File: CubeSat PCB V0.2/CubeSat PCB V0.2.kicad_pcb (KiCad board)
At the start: 2 copper layers, 34.4 x 65.5 mm, 8 parts, among them J1 Raspberry_Pi_2_3, J2 Encoder Connector, J3 LSM9DS1, J4 XT60PW-M, J5 Conn_01x03_Female, J6 XT60PW-F, SW1 SW_DPDT_x2, U1 MP1584EN

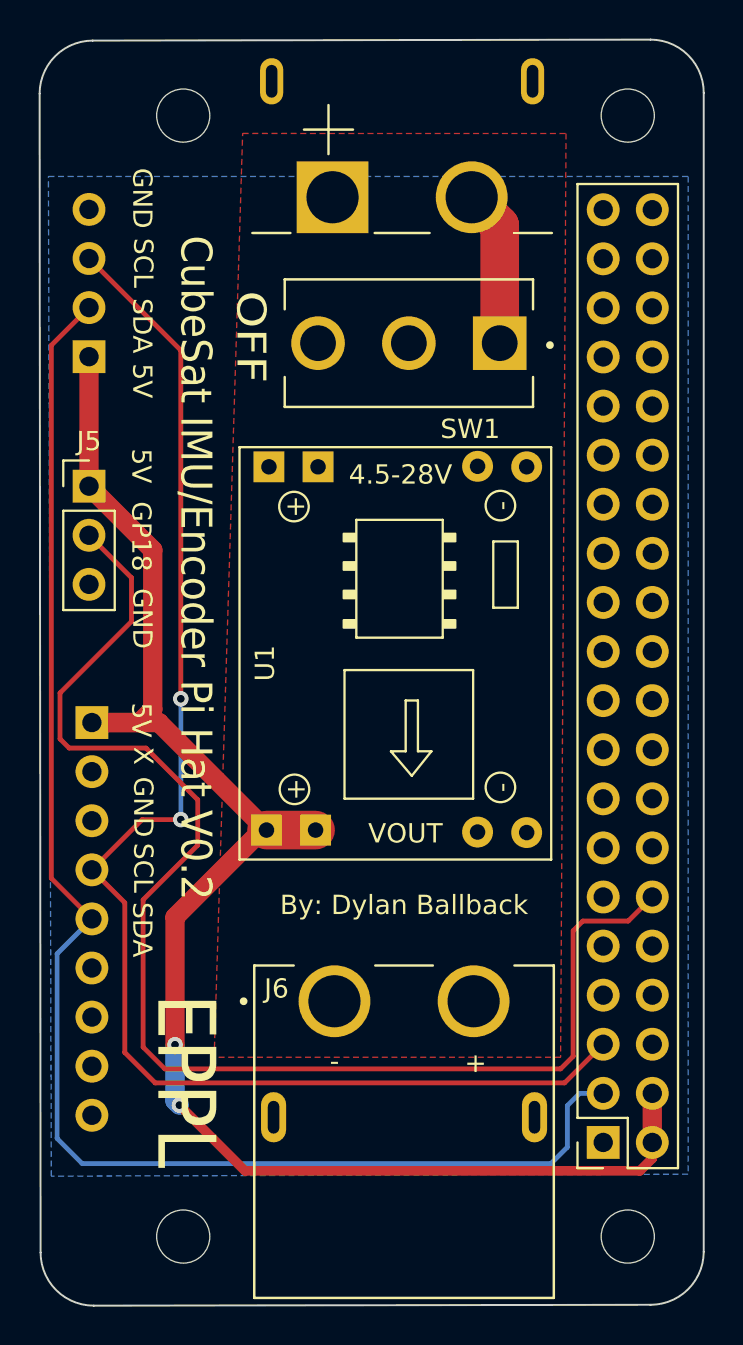
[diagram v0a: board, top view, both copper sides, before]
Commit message: Add files via upload
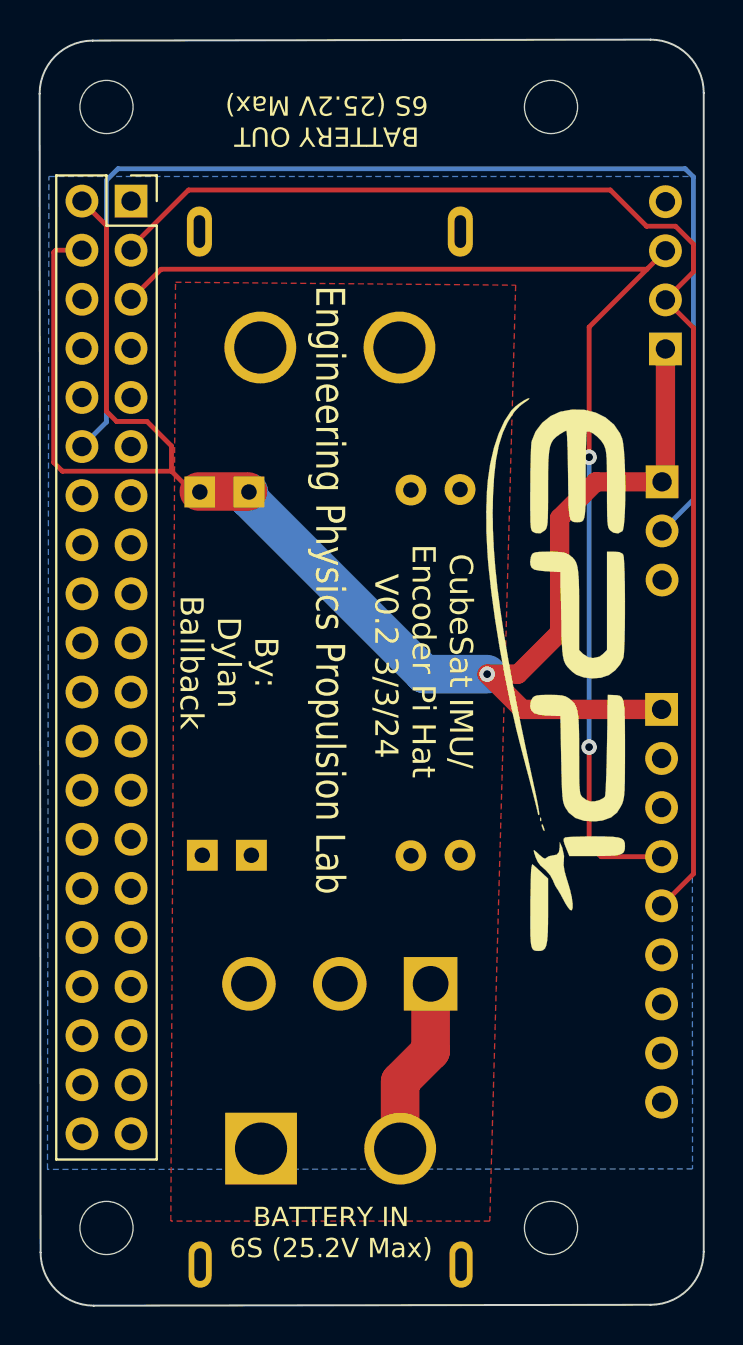
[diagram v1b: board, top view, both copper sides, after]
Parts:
- added G***: LOGO, dylan:eppl_logo2, F.Cu at (112.1, 95.1)
- J4, J5, J6, SW1, U1: moved to B.Cu
- moved J4 61.3 mm to (100.4, 125.4)
- moved J1 54.5 mm to (90.1, 70.3), turned to 0 degrees
- moved J6 34.0 mm to (100.4, 77.9)
- moved SW1 33.3 mm to (100.9, 110.8)
- moved J2 29.8 mm to (117.7, 78.0)
- moved J5 29.7 mm to (117.5, 84.9), turned to 180 degrees
- moved J3 29.5 mm to (117.5, 96.7)
- moved U1 3.45 mm to (100.9, 94.0), turned to 90 degrees
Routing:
- net /SCL: track 73.1 -> 63.7 mm
- net /SDA: track 77.0 -> 67.8 mm
- net +5V: track 82.9 -> 89.7 mm, vias 2 -> 1
- net /led: track 69.7 -> 64.1 mm
- net Net-(J4-Pad2): track 8.15 -> 9.18 mm
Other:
- board text added: "BATTERY IN 6S (25.2V Max)"
- board text added: "BATTERY OUT 6S (25.2V Max)"
- board text added: "CubeSat IMU/ Encoder Pi Hat V0.2 3/3/24"
- board text removed: "CubeSat IMU/Encoder Pi Hat V0.2 3/3/24"
